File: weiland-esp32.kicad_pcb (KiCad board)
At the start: 2 copper layers, 70.8 x 24.6 mm, 36 parts, among them J1 S02B-PASK-2, J6 S02B-PASK-2, J7 S02B-PASK-2, P1 S04B-PASK-2_LF__SN_, P2 S04B-PASK-2_LF__SN_, U1 ESP32-WROOM-32E(8MB), U2 AMS1117-3.3_C347222, U3 MAX98357AETE_T, U5 ULN2003F12FN-7, U6 DZ127S-22-06-55

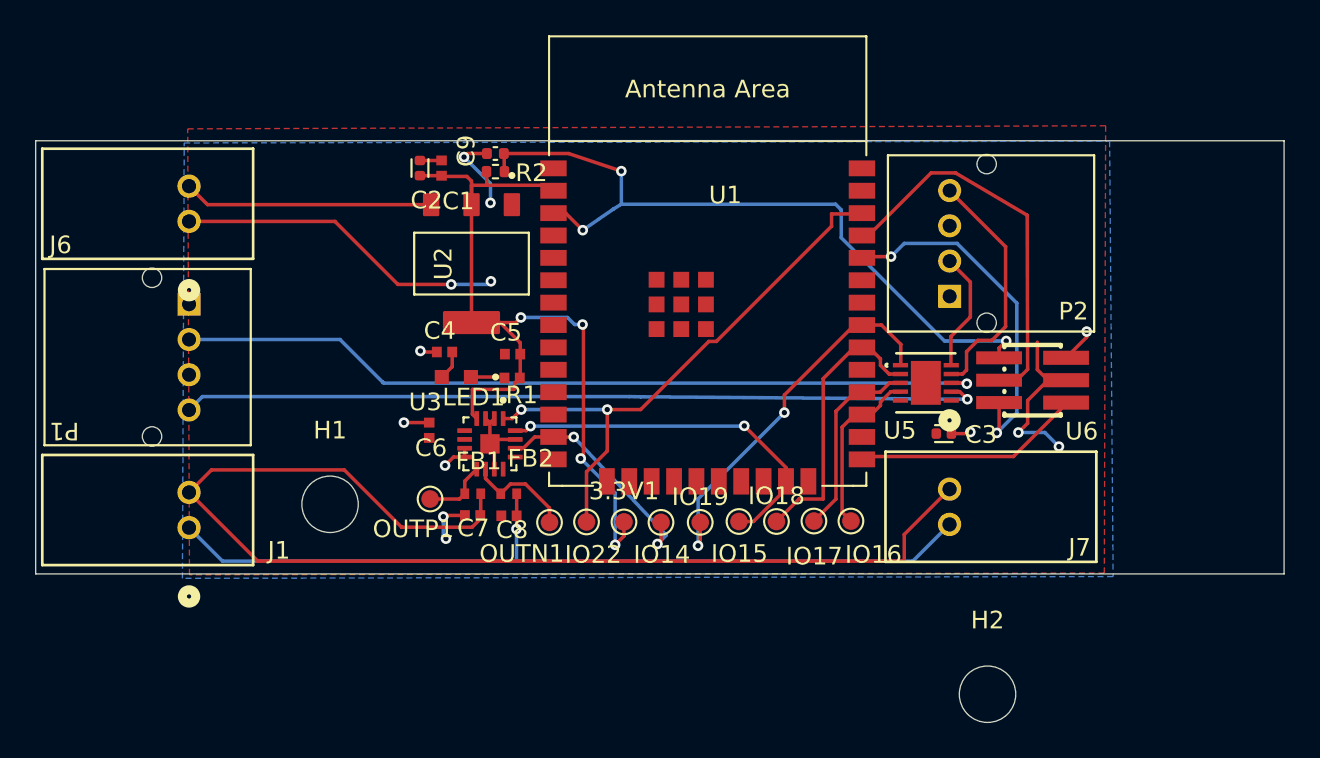
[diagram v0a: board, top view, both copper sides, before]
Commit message: board complete
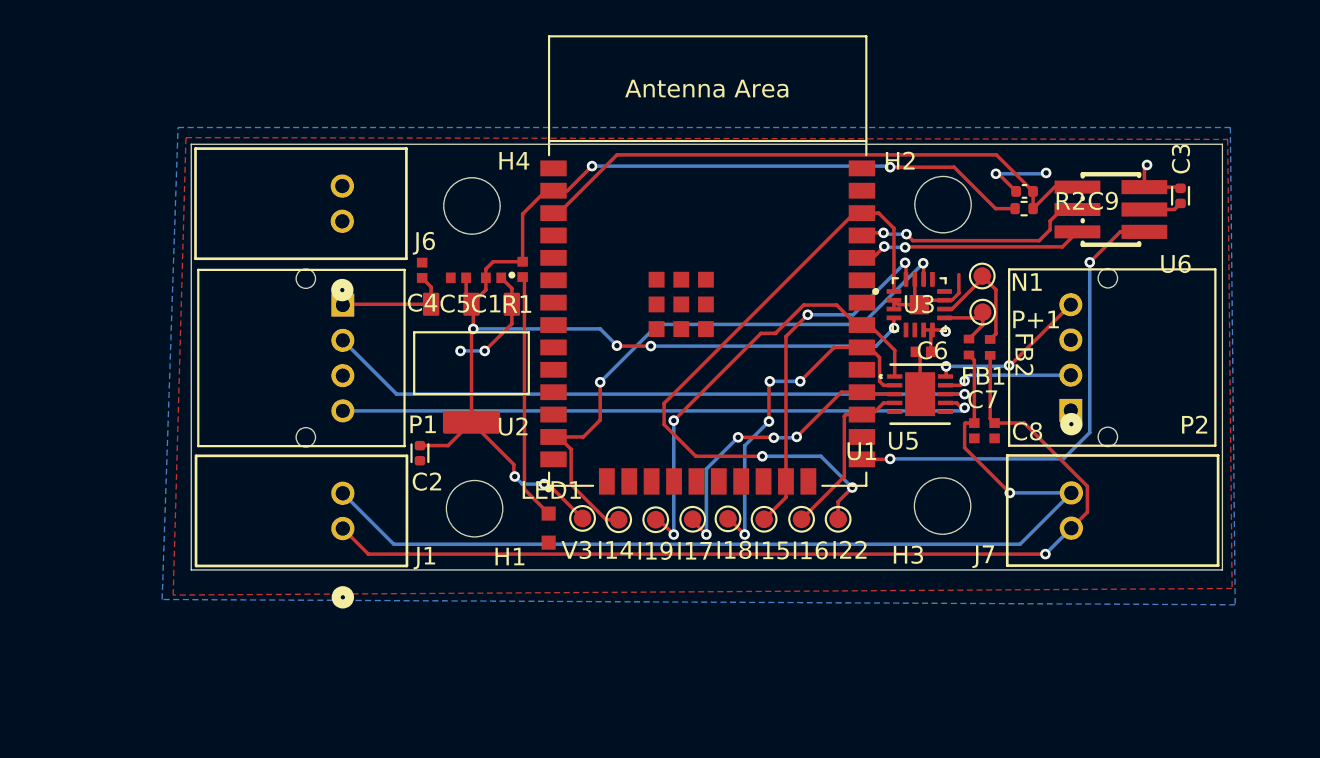
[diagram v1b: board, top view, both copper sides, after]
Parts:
- added H3: MountingHole, MountingHole:MountingHole_3.2mm_M3, F.Cu at (172.4, 108.4)
- added H4: MountingHole, MountingHole:MountingHole_3.2mm_M3, F.Cu at (145.7, 91.4)
- moved P+1 33.1 mm to (174.7, 97.4)
- moved C9 30.1 mm to (177.1, 90.5)
- moved R2 30.1 mm to (177.1, 91.5)
- moved FB1 29.4 mm to (173.9, 99.4), turned to -90 degrees
- moved C7 28.9 mm to (174.2, 104.1), turned to -90 degrees
- moved FB2 28.5 mm to (175.1, 99.4), turned to -90 degrees
- moved C6 28.4 mm to (171.3, 99.7), turned to 180 degrees
- moved N1 28.2 mm to (174.7, 95.3)
- moved C8 28.0 mm to (175.4, 104.1), turned to -90 degrees
- moved H2 27.9 mm to (172.4, 91.3)
- moved U3 25.6 mm to (171.1, 97.0), turned to 0 degrees
- moved C3 19.0 mm to (185.9, 90.8), turned to 90 degrees
- moved C2 16.2 mm to (142.8, 105.4), turned to 90 degrees
- moved I22 14.3 mm to (166.5, 109.2)
- moved U6 10.7 mm to (182.0, 91.6)
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- renumbered IO14 to I14, IO15 to I15, IO16 to I16, IO17 to I17, IO18 to I18, IO19 to I19, IO22 to I22, OUTN1 to N1, OUTP1 to P+1, 3.3V1 to V3
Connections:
- P2 pad 2: /OUTA -> /OUTB
- P2 pad 4: /OUTB -> /OUTA
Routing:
- net +3.3V: track 49.5 -> 83.5 mm, vias 4 -> 8
- net GND: track 43.5 -> 22.3 mm, vias 8 -> 4
- net /IO14: track 13.3 -> 34.1 mm
- net /IO0: track 13.0 -> 27.0 mm, vias 0 -> 2
- net Net-(LED1-A): track 1.93 -> 14.0 mm
- net /OUTP: track 67.4 -> 56.8 mm, vias 0 -> 1
- net /OUTD: track 45.6 -> 36.5 mm
- net +5V: track 21.6 -> 12.7 mm, vias 5 -> 2
- net /TXD0: track 22.1 -> 13.5 mm, vias 0 -> 2
- net /OUTC: track 46.1 -> 37.6 mm
- net /EN: track 41.5 -> 33.4 mm, vias 3 -> 0
- net /OUTN: track 48.6 -> 56.0 mm
- net /RXD0: track 20.1 -> 12.9 mm
- net /OUTB: track 13.8 -> 7.35 mm, vias 0 -> 1
- net /IO17: track 11.1 -> 17.5 mm, vias 0 -> 4
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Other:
- board size 70.8 x 24.6 mm -> 58.5 x 24.2 mm
